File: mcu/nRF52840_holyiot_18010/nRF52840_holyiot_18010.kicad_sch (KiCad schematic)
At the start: 3 parts

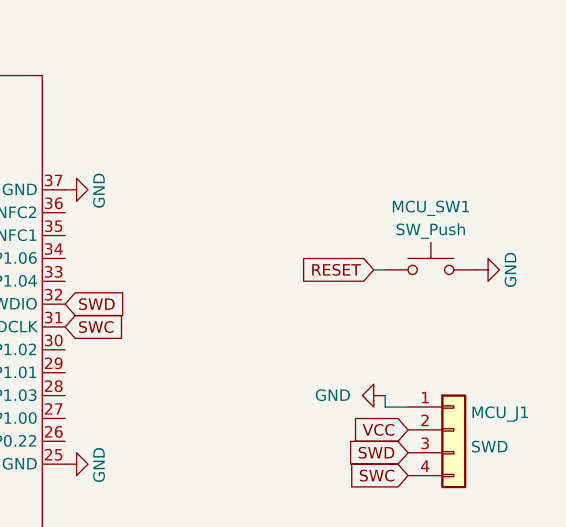
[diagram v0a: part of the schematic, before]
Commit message: add reset module
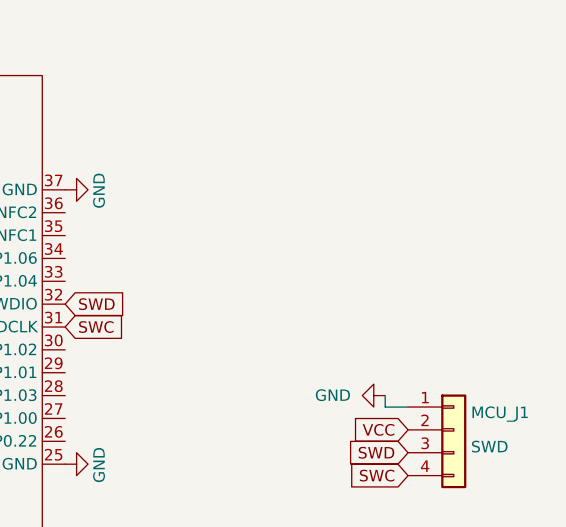
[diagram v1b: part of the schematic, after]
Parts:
- removed MCU_SW1: SW_Push, ErgoCai.pretty:K2-1187SQ, symbol Switch:SW_Push
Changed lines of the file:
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@@
-		)
-	)
-	(wire
-		(pts
-			(xy 143.51 54.61) (xy 144.78 54.61)
-		)
-		(stroke
-			(width 0)
-			(type solid)
 		)
 	)
@@
 		(property "Intersheetrefs" "${INTERSHEET_REFS}"
 			(at 90.17 97.6303 90)
-			(effects
-				(font
-					(size 1.27 1.27)
-				)
-				(justify right)
-				(hide yes)
-			)
-		)
-	)
-	(global_label "RESET"
-		(shape input)
-		(at 143.51 54.61 180)
-		(fields_autoplaced yes)
-		(effects
-			(font
-				(size 1.27 1.27)
-			)
-			(justify right)
-		)
-		(property "Intersheetrefs" "${INTERSHEET_REFS}"
-			(at 134.7797 54.61 0)
 			(effects
 				(font
@@
 					(unit 1)
 				)
-			)
-		)
-	)
-	(symbol
-		(lib_id "power:GND")
-		(at 154.94 54.61 90)
-		(unit 1)
-		(exclude_from_sim no)
-		(in_bom yes)
-		(on_board yes)
-		(dnp no)
-		(property "Reference" "#PWR0103"
-			(at 161.29 54.61 0)
-			(effects
-				(font
-					(size 1.27 1.27)
-				)
-				(hide yes)
-			)
-		)
-		(property "Value" "GND"
-			(at 158.75 54.61 0)
-			(effects
-				(font
-					(size 1.27 1.27)
-				)
-			)
-		)
-		(property "Footprint" ""
-			(at 154.94 54.61 0)
-			(effects
-				(font
-					(size 1.27 1.27)
-				)
-				(hide yes)
-			)
-		)
-		(property "Datasheet" ""
-			(at 154.94 54.61 0)
-			(effects
-				(font
-					(size 1.27 1.27)
-				)
-				(hide yes)
-			)
-		)
-		(property "Description" "Power symbol creates a global label with name \"GND\" , ground"
-			(at 154.94 54.61 0)
-			(effects
-				(font
-					(size 1.27 1.27)
-				)
-				(hide yes)
-			)
-		)
-		(pin "1"
-		)
-		(instances
-			(project "nRF52840_holyiot_18010"
-				(path "/a75e1a70-312e-4b3d-9ad5-017ab62e82c1"
-					(reference "#PWR0103")
-					(unit 1)
-				)
-			)
-		)
-	)
-	(symbol
-		(lib_id "Switch:SW_Push")
-		(at 149.86 54.61 0)
-		(unit 1)
-		(exclude_from_sim no)
-		(in_bom yes)
-		(on_board yes)
-		(dnp no)
-		(property "Reference" "MCU_SW1"
-			(at 149.86 47.625 0)
-			(effects
-				(font
-					(size 1.27 1.27)
-				)
-			)
-		)
-		(property "Value" "SW_Push"
-			(at 149.86 50.165 0)
-			(effects
-				(font
-					(size 1.27 1.27)
-				)
-			)
-		)
-		(property "Footprint" "ErgoCai.pretty:K2-1187SQ"
-			(at 149.86 49.53 0)
-			(effects
-				(font
-					(size 1.27 1.27)
-				)
-				(hide yes)
-			)
-		)
-		(property "Datasheet" "~"
-			(at 149.86 49.53 0)
-			(effects
-				(font
-					(size 1.27 1.27)
-				)
-				(hide yes)
-			)
-		)
-		(property "Description" "Push button switch, generic, two pins"
-			(at 149.86 54.61 0)
-			(effects
-				(font
-					(size 1.27 1.27)
-				)
-				(hide yes)
-			)
-		)
-		(pin "1"
-		)
-		(pin "2"
-		)
-		(instances
-			(project "nRF52840_holyiot_18010"
-				(path "/a75e1a70-312e-4b3d-9ad5-017ab62e82c1"
-					(reference "MCU_SW1")
-					(unit 1)
-				)
